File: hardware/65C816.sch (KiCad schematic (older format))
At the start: 25 parts, among them J1 POWER, U1 74AC00, U2 W65C816SxP, U3 74AC245, U4 74AC573, U5 74AC04

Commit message: Update for episode 6
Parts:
- removed unit 2 of U1
- removed U5: 74AC04, symbol 74xx:74LS04
- added C10, C11: 100n, symbol Device:C_Small
- added unit 3 of U1
- added U6: 74AC74, symbol 74xx:74LS74
- added U8: 74AC08, symbol 74xx:74LS08
- added U9: 74AC32, symbol 74xx:74LS32
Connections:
- net labels added: CLK*2, ~CLK
- wire segments 151 -> 191
- no-connect marks 10 -> 13
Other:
- moved on the sheet: D2, R2, RN1, RN2, RN3, RN4, RN5, RN6, U1D, U1E, U2, U3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

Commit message: Updates for episode 7
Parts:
- removed U8: 74AC08, symbol 74xx:74LS08
- added C12: 100n, symbol Device:C_Small
- added U5: DS1035-10, symbol 65C816:DS1035-10
- added U8: 74AC11, symbol 74xx:74LS11
- U3: value 74AC245 -> 74ACT245
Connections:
- wire segments 191 -> 199
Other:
- moved on the sheet: C1, C10, C11, C2, C3, C4, C5, C6, C7, C8, C9, D1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

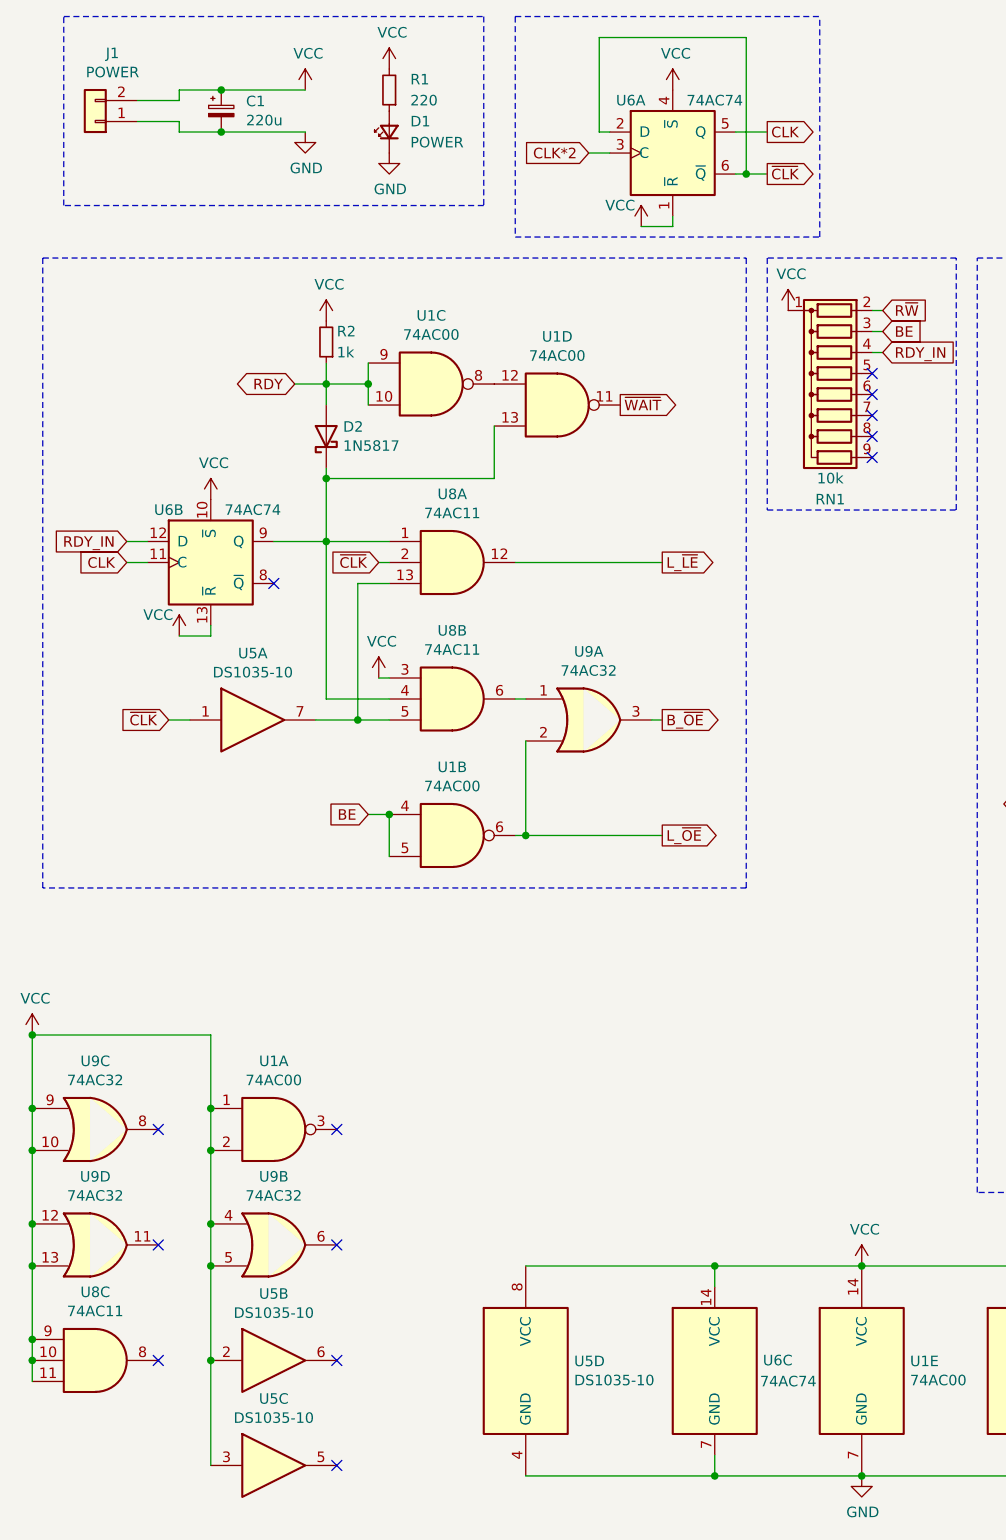
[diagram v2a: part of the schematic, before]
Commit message: Updates for episode 8
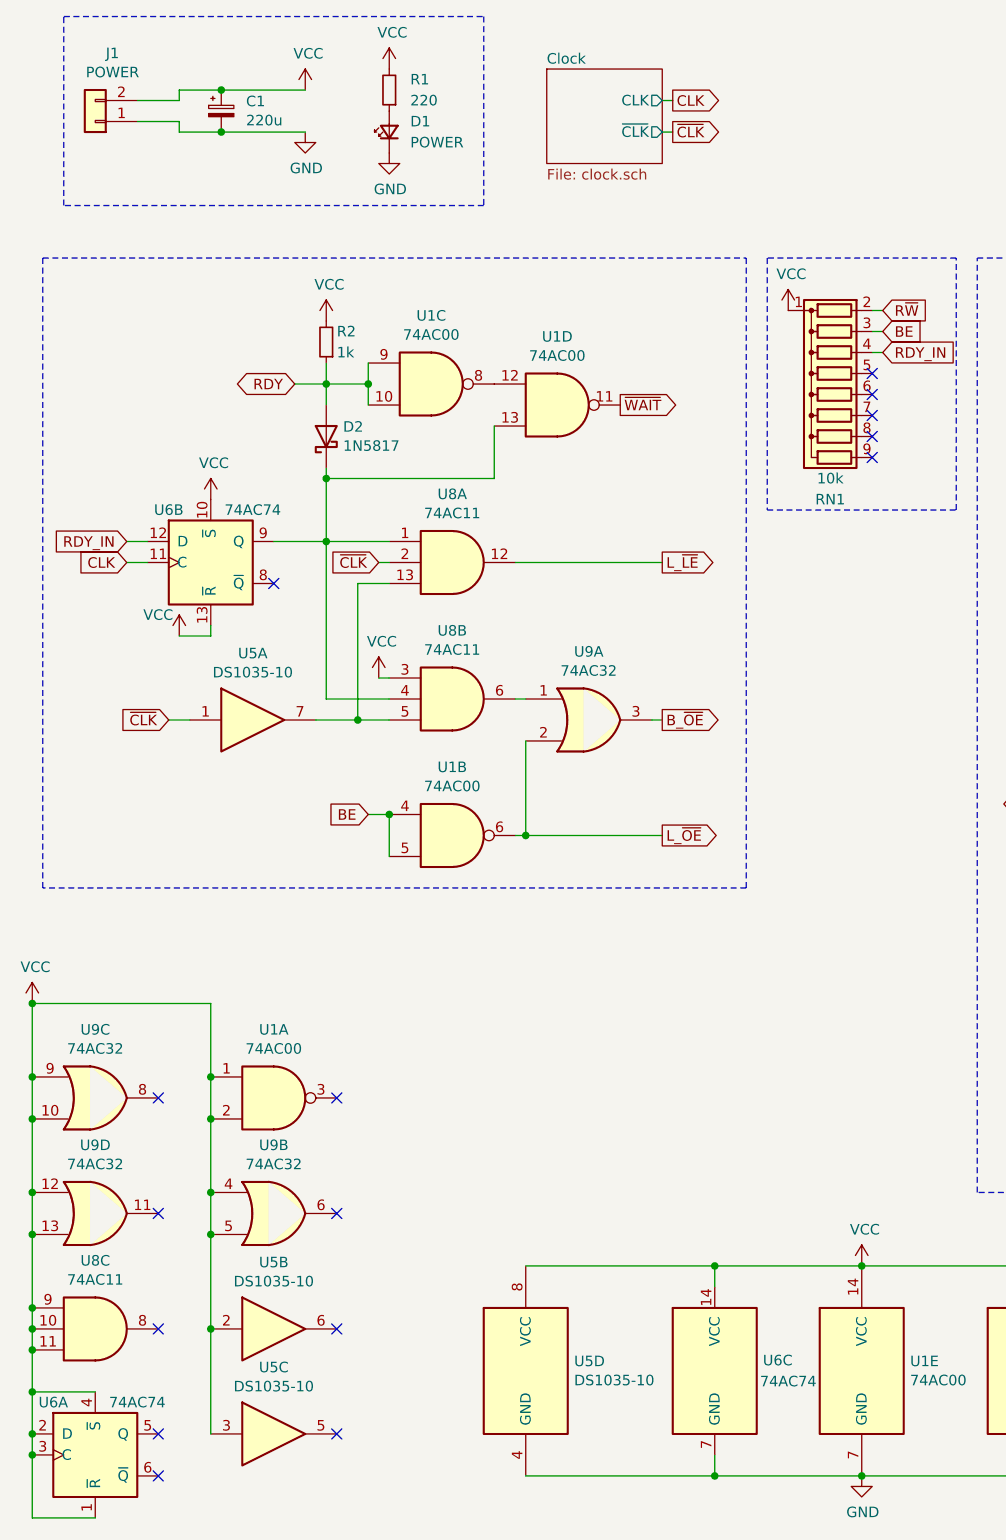
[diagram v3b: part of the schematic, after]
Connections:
- net CLK*2 is gone; now on net VCC: U6.3 (C)
- net CLK: no longer U6.5 (Q)
- net VCC: now also U6.2 (D)
- net ~CLK: no longer U6.2 (D), U6.6 (~Q)
- no-connect marks 13 -> 15
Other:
- moved on the sheet: U1A, U5B, U5C, U6A, U8C, U9B, U9C, U9D

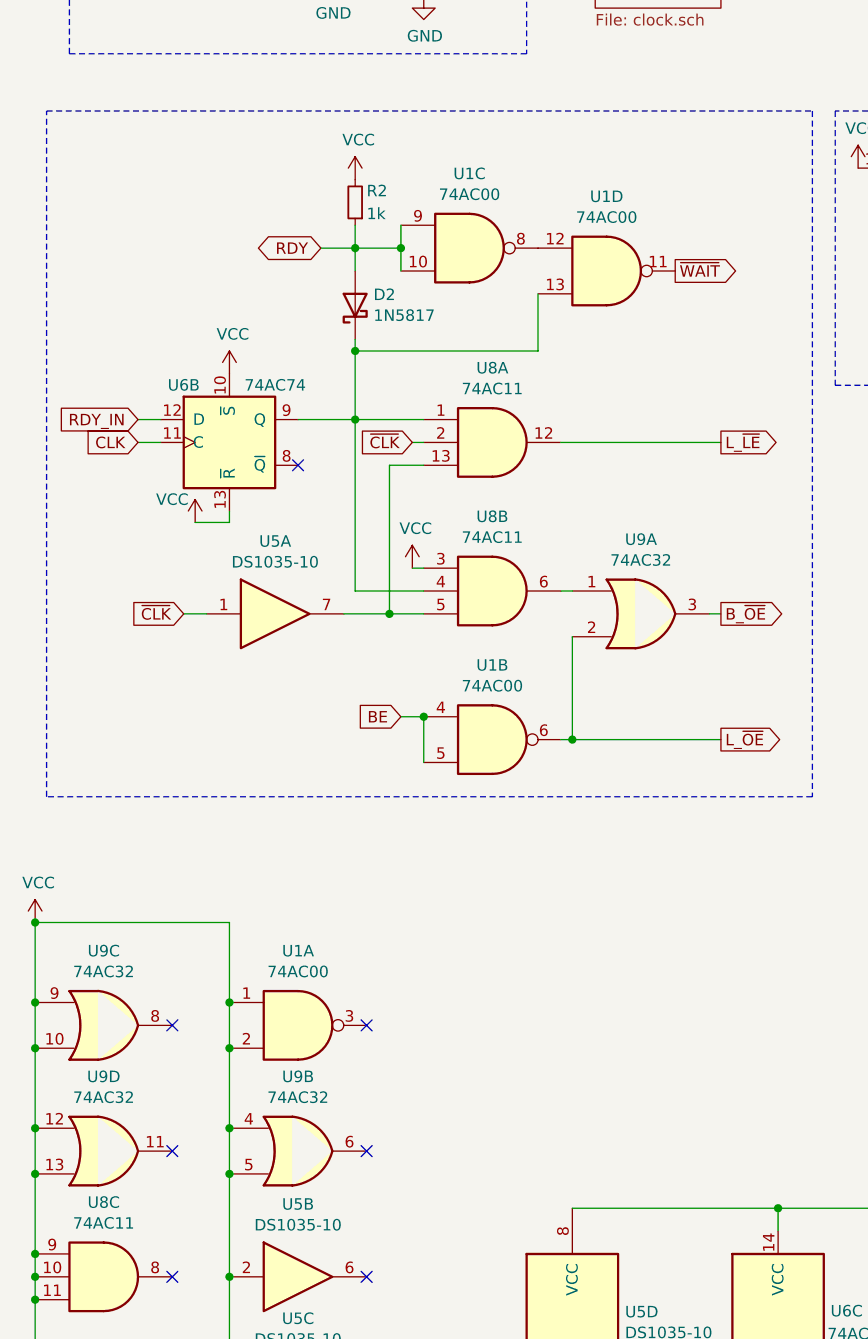
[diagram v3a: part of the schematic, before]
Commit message: Updates for episode 9
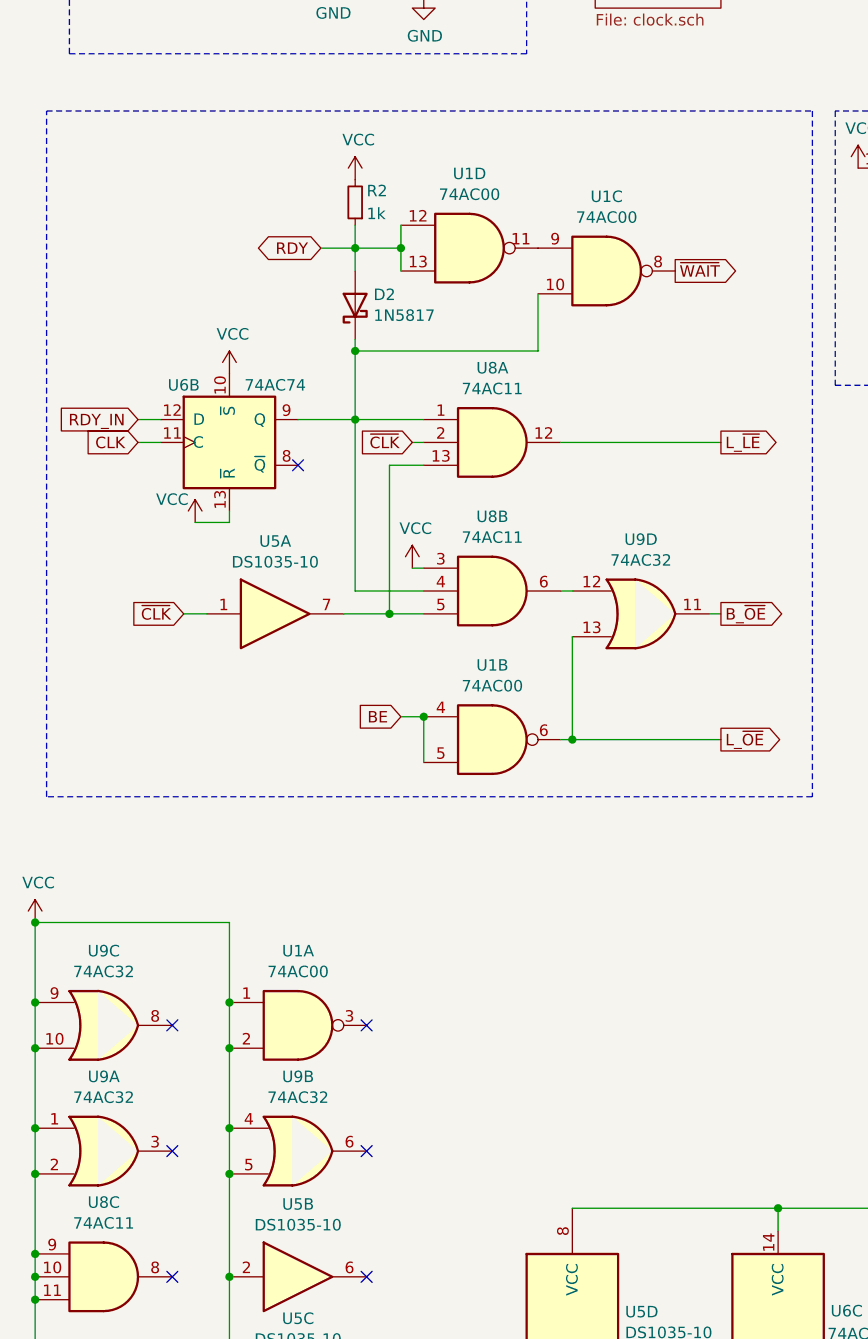
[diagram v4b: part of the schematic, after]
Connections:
- net B_~OE: now also U9.11; no longer U9.3
- net L_~OE: now also U9.13; no longer U9.2
- net RDY: now also U1.12, U1.13; no longer U1.10, U1.9
- net VCC: now also U9.1, U9.2; no longer U9.12, U9.13
- net ~WAIT: now also U1.8; no longer U1.11
- net at D2.1 (K), U6.9 (Q), U8.1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: now also U1.10; no longer U1.13
- net at U8.6: now also U9.12; no longer U9.1
- new net: U1.11, U1.9
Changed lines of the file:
@@
 $Comp
 L 74xx:74LS32 U9
-U 4 1 6186BC0D
+U 1 1 6186BC0D
 P 900 6300
 F 0 "U9" H 900 6625 50  0000 C CNN
@@
 F 2 "" H 900 6300 50  0001 C CNN
 F 3 "https://www.ti.com/lit/ds/symlink/sn54ac32.pdf" H 900 6300 50  0001 C CNN
-	4    900  6300
+	1    900  6300
 	1    0    0    -1
 $EndComp
@@
 $Comp
 L 74xx:74HC00 U1
-U 3 1 617F2205
+U 4 1 617F2205
 P 2500 2350
 F 0 "U1" H 2500 2675 50  0000 C CNN
@@
 F 2 "" H 2500 2350 50  0001 C CNN
 F 3 "https://www.ti.com/lit/ds/symlink/sn74ac00.pdf" H 2500 2350 50  0001 C CNN
-	3    2500 2350
+	4    2500 2350
 	1    0    0    -1
 $EndComp
@@
 $Comp
 L 74xx:74LS32 U9
-U 1 1 6161DFB3
+U 4 1 6161DFB3
 P 3250 3950
 F 0 "U9" H 3250 4275 50  0000 C CNN
@@
 F 2 "" H 3250 3950 50  0001 C CNN
 F 3 "https://www.ti.com/lit/ds/symlink/sn54ac32.pdf" H 3250 3950 50  0001 C CNN
-	1    3250 3950
+	4    3250 3950
 	1    0    0    -1
 $EndComp
@@
 $Comp
 L 74xx:74HC00 U1
-U 4 1 610F744F
+U 3 1 610F744F
 P 3100 2450
 F 0 "U1" H 3100 2775 50  0000 C CNN
@@
 F 2 "" H 3100 2450 50  0001 C CNN
 F 3 "https://www.ti.com/lit/ds/symlink/sn74ac00.pdf" H 3100 2450 50  0001 C CNN
-	4    3100 2450
+	3    3100 2450
 	1    0    0    -1
 $EndComp
